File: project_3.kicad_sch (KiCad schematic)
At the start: 20 parts, among them SW1 SW_Push, SW2 SW_Push, SW3 SW_Push, U1 LPC2148FBD64, Y1 12MHz

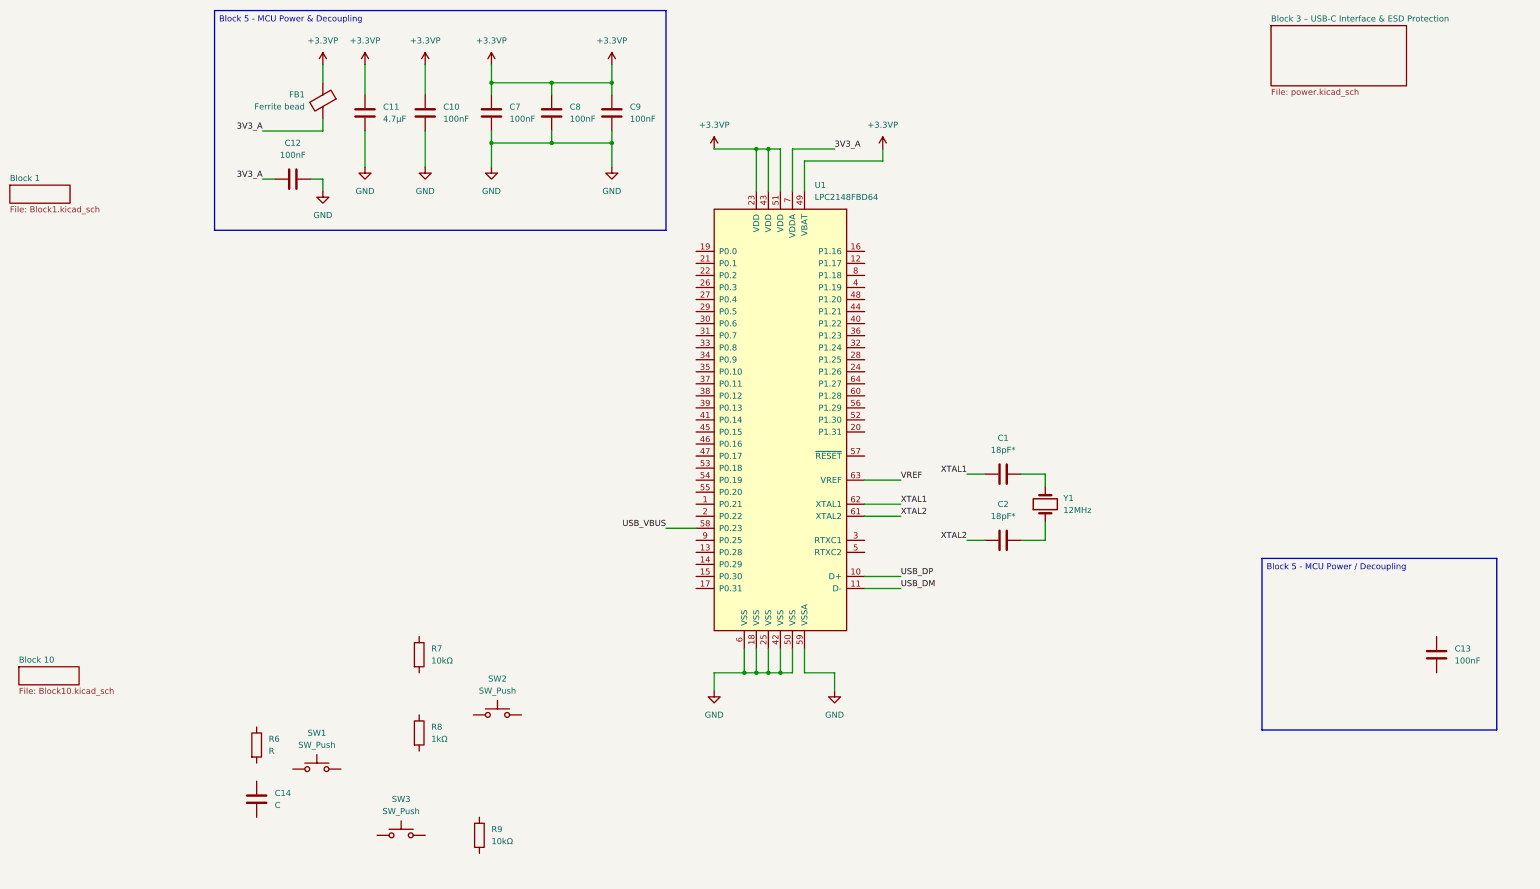
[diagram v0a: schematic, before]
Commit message: ports added
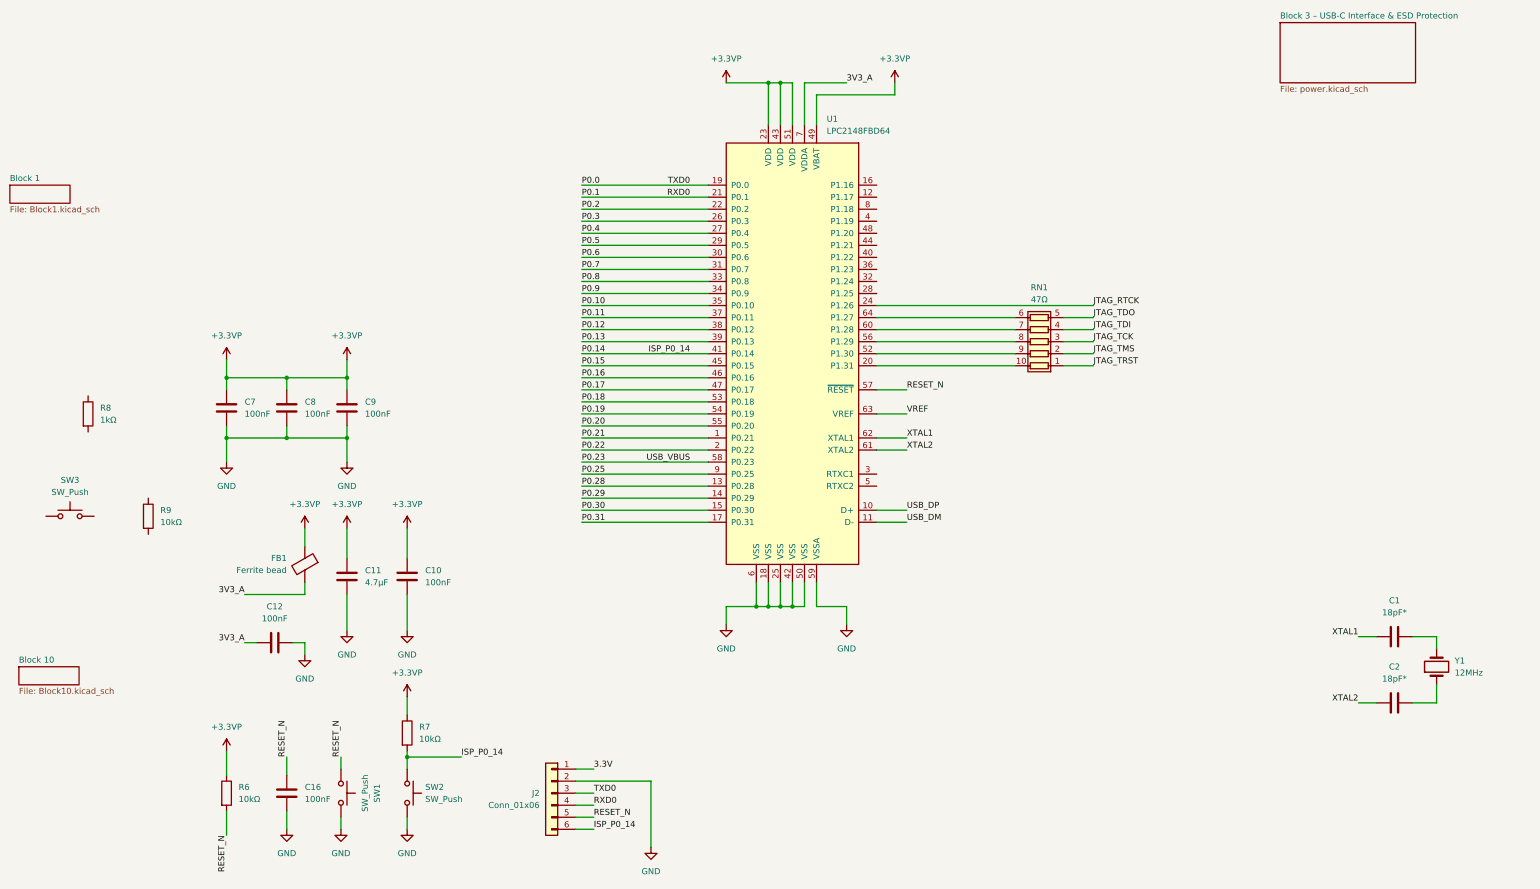
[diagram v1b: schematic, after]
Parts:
- removed C13: 100nF, Capacitor_SMD:C_0603_1608Metric, symbol Device:C
- removed C14: C, Capacitor_SMD:C_0603_1608Metric, symbol Device:C
- added C16: 100nF, Capacitor_SMD:C_0603_1608Metric, symbol Device:C
- added J2: Conn_01x06, Connector_PinHeader_2.54mm:PinHeader_1x06_P2.54mm_Vertical, symbol Connector_Generic:Conn_01x06
- added RN1: 47Ω, Resistor_THT:R_Array_SIP14, symbol Device:R_Pack05
- R6: value R -> 10kΩ
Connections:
- net +3.3VP: now also R6.1, R7.1
- net GND: now also SW1.1, SW2.2, C16.2, J2.2 (Pin_2)
- net P0.21: now reaches U1.1 (P0.21)
- net P0.28: now reaches U1.13 (P0.28)
- net P0.29: now reaches U1.14 (P0.29)
- net P0.30: now reaches U1.15 (P0.30)
- net P0.31: now reaches U1.17 (P0.31)
- net P0.0: now reaches U1.19 (P0.0)
- net P0.0: now also J2.3 (Pin_3)
- net P0.22: now reaches U1.2 (P0.22)
- net at U1.20 (P1.31): now also RN1.10 (R1.2)
- net P0.1: now reaches U1.21 (P0.1)
- net P0.1: now also J2.4 (Pin_4)
- net P0.2: now reaches U1.22 (P0.2)
- net JTAG_RTCK: now reaches U1.24 (P1.26)
- net P0.3: now reaches U1.26 (P0.3)
- net P0.4: now reaches U1.27 (P0.4)
- net P0.5: now reaches U1.29 (P0.5)
- net P0.6: now reaches U1.30 (P0.6)
- net P0.7: now reaches U1.31 (P0.7)
- net P0.8: now reaches U1.33 (P0.8)
- net P0.9: now reaches U1.34 (P0.9)
- net P0.10: now reaches U1.35 (P0.10)
- net P0.11: now reaches U1.37 (P0.11)
- net P0.12: now reaches U1.38 (P0.12)
- net P0.13: now reaches U1.39 (P0.13)
- net ISP_P0_14: now reaches U1.41 (P0.14)
- net ISP_P0_14: now also R7.2, SW2.1, J2.6 (Pin_6)
- net P0.15: now reaches U1.45 (P0.15)
- net P0.16: now reaches U1.46 (P0.16)
- net P0.17: now reaches U1.47 (P0.17)
- net at U1.52 (P1.30): now also RN1.9 (R2.2)
- net P0.18: now reaches U1.53 (P0.18)
- net P0.19: now reaches U1.54 (P0.19)
- net P0.20: now reaches U1.55 (P0.20)
- net at U1.56 (P1.29): now also RN1.8 (R3.2)
- net RESET_N: now reaches U1.57 (~{RESET})
- net RESET_N: now also R6.2, SW1.2, C16.1, J2.5 (Pin_5)
- net at U1.60 (P1.28): now also RN1.7 (R4.2)
- net at U1.64 (P1.27): now also RN1.6 (R5.2)
- net P0.25: now reaches U1.9 (P0.25)
- net USB_VBUS renamed P0.23
- new net 3.3V: J2.1 (Pin_1)
- new net JTAG_TCK: RN1.3 (R3.1)
- new net JTAG_TDI: RN1.4 (R4.1)
- new net JTAG_TDO: RN1.5 (R5.1)
- new net JTAG_TMS: RN1.2 (R2.1)
- new net JTAG_TRST: RN1.1 (R1.1)
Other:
- moved on the sheet: C1, C10, C11, C12, C2, C7, C8, C9, FB1, R6, R7, R8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
